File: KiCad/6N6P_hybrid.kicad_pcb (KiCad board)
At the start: 2 copper layers, 170 x 140.9 mm, 71 parts, among them J1 MID Select, J10 Screw_Terminal_01x03, J11 Screw_Terminal_01x01, J12 Screw_Terminal_01x01, J13 Screw_Terminal_01x01, J14 Screw_Terminal_01x01, J15 PSU ground, J16 Screw_Terminal_01x01, J17 center tap, J18 chassis, J2 Input, J3 MID Bypass, J4 Low boost, J5 PrePower, J6 Volume, J7 Hi Cut, J8 6N6P, J9 OT feedback, Q1 BC107, U1 LTC1151CN8, U2 LTC1151CN8

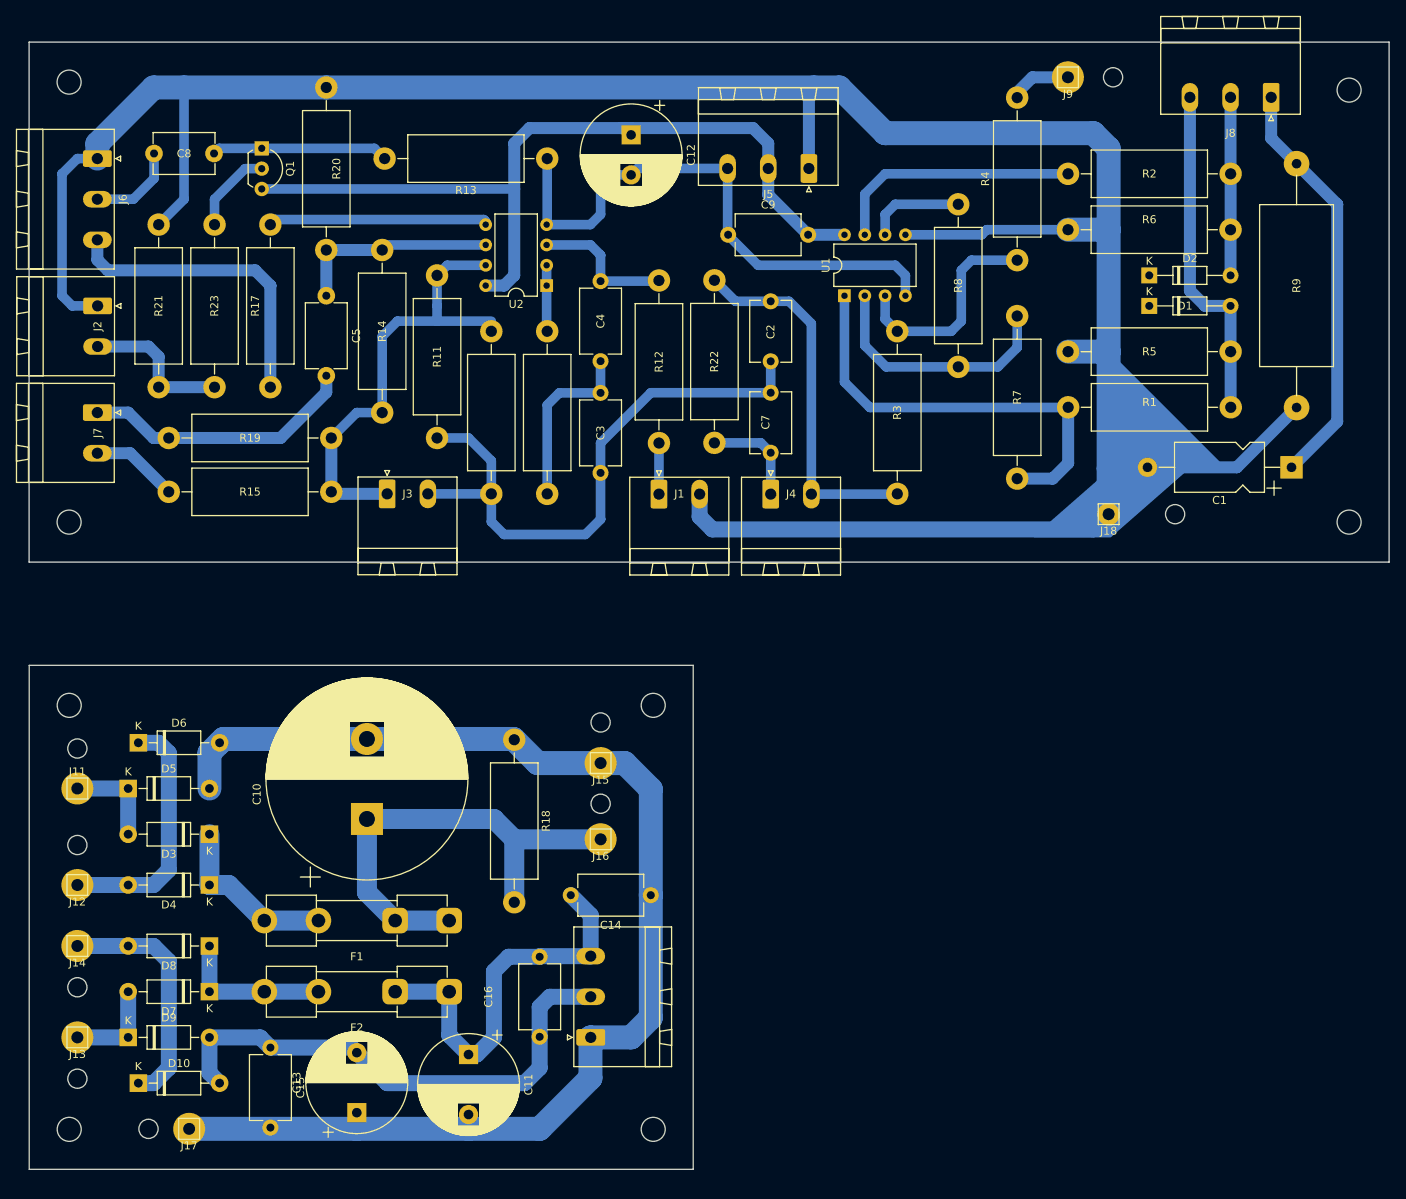
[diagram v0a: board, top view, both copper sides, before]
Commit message: Add files via upload
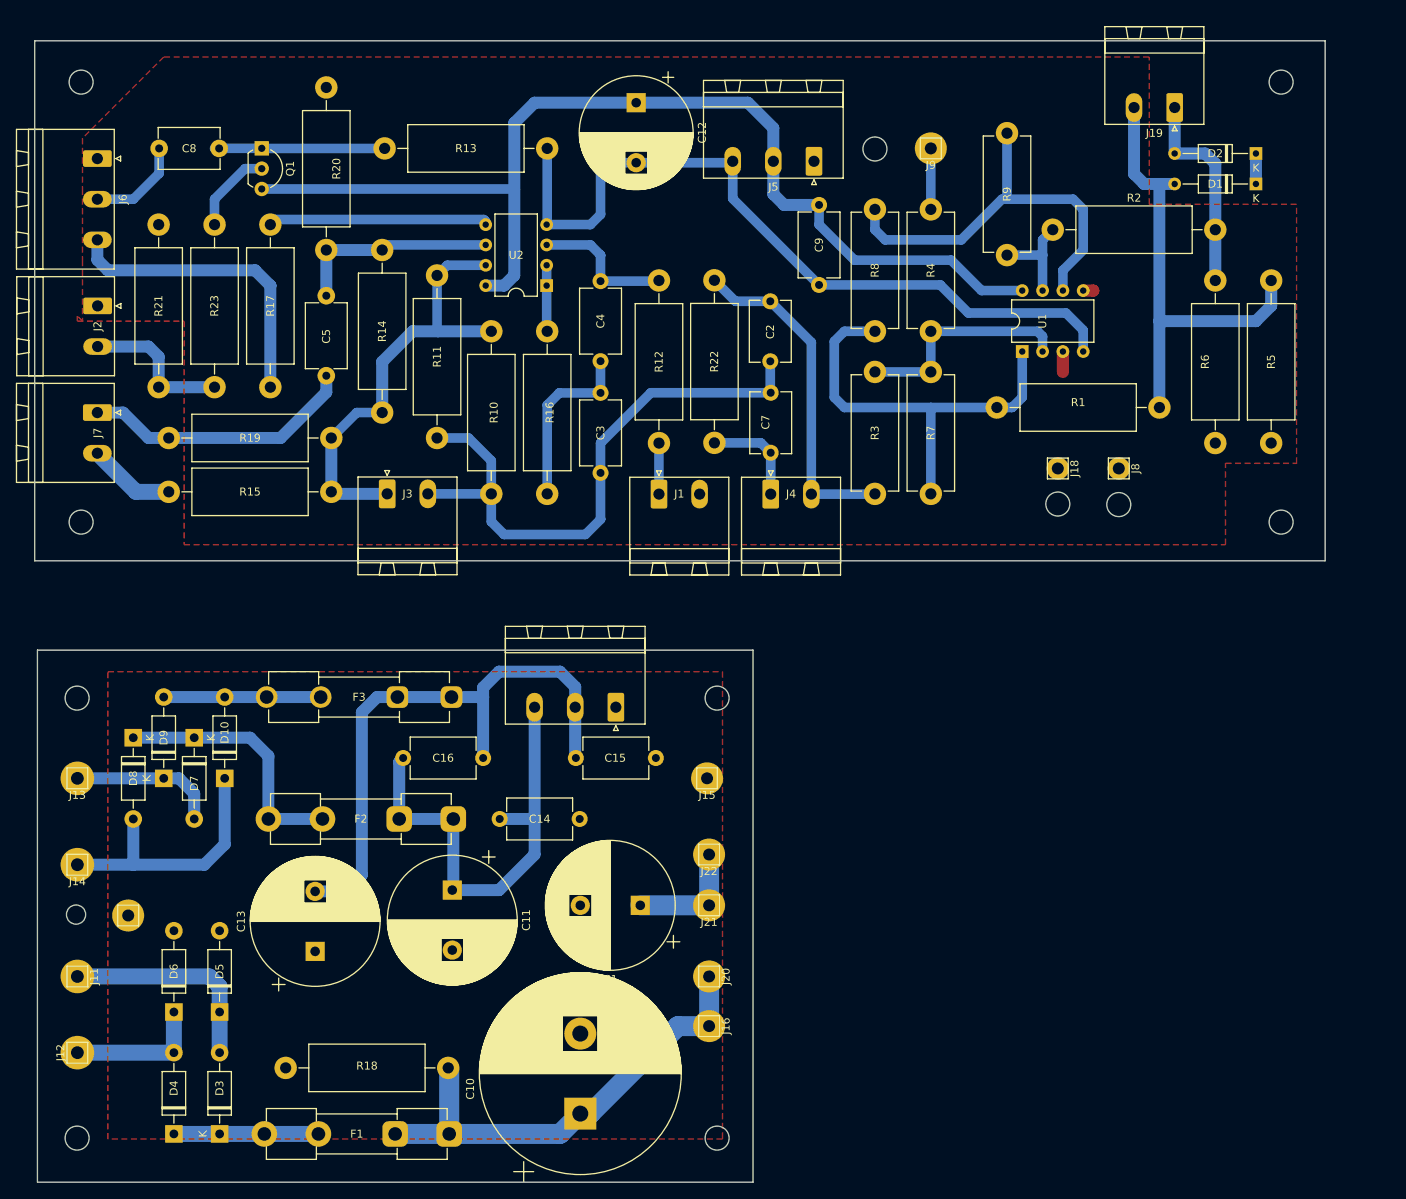
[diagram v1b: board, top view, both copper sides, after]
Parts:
- added F3: Fuse, Fuse:Fuseholder_Clip-5x20mm_Keystone_3517_Inline_P23.11x6.76mm_D1.70mm_Horizontal, F.Cu at (72.8, 102.9)
- added J19: TUBE, Connector_Phoenix_MSTB:PhoenixContact_MSTBA_2,5_2-G-5,08_1x02_P5.08mm_Horizontal, F.Cu at (163.2, 29.2)
- added J20: Screw_Terminal_01x01, Connector_Pin:Pin_D1.1mm_L8.5mm_W2.5mm_FlatFork, F.Cu at (105.0, 137.8)
- added J21: Screw_Terminal_01x01, Connector_Pin:Pin_D1.1mm_L8.5mm_W2.5mm_FlatFork, F.Cu at (105.0, 128.9)
- added J22: Screw_Terminal_01x01, Connector_Pin:Pin_D1.1mm_L8.5mm_W2.5mm_FlatFork, F.Cu at (105.0, 122.6)
- C1: value 22u -> 68u/350V; footprint Capacitor_THT:CP_Axial_L11.0mm_D6.0mm_P18.00mm_Horizontal -> Capacitor_THT:CP_Radial_D16.0mm_P7.50mm
- C11, C13: footprint Capacitor_THT:CP_Radial_D12.5mm_P7.50mm -> Capacitor_THT:CP_Radial_D16.0mm_P7.50mm
- C12: footprint Capacitor_THT:CP_Radial_D12.5mm_P5.00mm -> Capacitor_THT:CP_Radial_D14.0mm_P7.50mm
- J8: value 6N6P -> chassis; footprint Connector_Phoenix_MSTB:PhoenixContact_MSTBA_2,5_3-G-5,08_1x03_P5.08mm_Horizontal -> Connector_Pin:Pin_D1.1mm_L8.5mm_W2.5mm_FlatFork
- R3, R4, R7: footprint Resistor_THT:R_Axial_DIN0614_L14.3mm_D5.7mm_P20.32mm_Horizontal -> Resistor_THT:R_Axial_DIN0614_L14.3mm_D5.7mm_P15.24mm_Horizontal
- R8: value 12k -> 10k; footprint Resistor_THT:R_Axial_DIN0614_L14.3mm_D5.7mm_P20.32mm_Horizontal -> Resistor_THT:R_Axial_DIN0614_L14.3mm_D5.7mm_P15.24mm_Horizontal
- R9: value 390, 5W -> 10k; footprint Resistor_THT:R_Axial_DIN0922_L20.0mm_D9.0mm_P30.48mm_Horizontal -> Resistor_THT:R_Axial_DIN0614_L14.3mm_D5.7mm_P15.24mm_Horizontal
- moved C1 98.1 mm to (96.4, 128.9)
- moved C15 52.6 mm to (88.3, 110.5), turned to 0 degrees
- moved J8 50.1 mm to (156.2, 74.3), turned to 90 degrees
- moved R18 50.0 mm to (52.1, 149.2), turned to 0 degrees
- moved R9 49.9 mm to (142.2, 32.4), turned to -90 degrees
- moved C10 45.5 mm to (88.9, 154.9)
- moved J10 41.4 mm to (93.3, 104.1), turned to 180 degrees
- moved D10 39.6 mm to (44.5, 113.0), turned to 90 degrees
- moved D3 37.5 mm to (43.8, 157.5), turned to 90 degrees
- moved C16 35.6 mm to (76.8, 110.5), turned to 180 degrees
- moved D6 33.9 mm to (38.1, 142.2), turned to 90 degrees
- moved D9 32.7 mm to (36.8, 113.0), turned to 90 degrees
- moved R6 32.4 mm to (168.3, 71.1), turned to 90 degrees
- moved J13 32.4 mm to (26.0, 113.0)
- moved D7 31.8 mm to (40.6, 108.0), turned to -90 degrees
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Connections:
- C1 pad 1: Net-(J8-Pin_1) -> Net-(J21-Pin_1)
- C1 pad 2: GND -> GND2
- C13 pad 2: Net-(D10-A) -> Net-(J10-Pin_2)
- C15 pad 1: Net-(D10-A) -> Net-(J10-Pin_2)
- C16 pad 1: Net-(D10-A) -> Net-(J10-Pin_2)
- J10 pad 2: Net-(D10-A) -> Net-(J10-Pin_2)
- J8 pad 1: Net-(J8-Pin_1) -> GND
- R3 pad 1: Net-(U1A-+) -> Net-(U1A--)
- R4 pad 1: Net-(U1A-+) -> Net-(U1A--)
- R8 pad 1: Net-(U1A--) -> Net-(U1B--)
- R8 pad 2: Net-(U1B--) -> Net-(R1-Pad1)
- R9 pad 1: GND -> Net-(U1B--)
- R9 pad 2: Net-(J8-Pin_1) -> Net-(R2-Pad1)
- U1 pad 3: Net-(U1A-+) -> GND
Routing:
- net GND: track 347.1 -> 3.82 mm
- net GND2: track 161.7 -> 0.00 mm
- net Net-(J10-Pin_2): track 0.00 -> 73.9 mm
- net Net-(J8-Pin_1): track 52.0 -> 0.00 mm
- net Net-(D10-A): track 65.2 -> 19.6 mm
- net Net-(U1B--): track 12.2 -> 51.2 mm
- net V++: track 105.7 -> 135.3 mm
- net Net-(U1A-+): track 27.7 -> 0.00 mm
- net V--: track 71.2 -> 95.8 mm
- net Net-(R2-Pad1): track 31.5 -> 12.6 mm
- net Net-(D1-A): track 42.7 -> 59.8 mm
- net Net-(J21-Pin_1): track 0.00 -> 14.9 mm
- net Net-(D3-A): track 12.1 -> 26.6 mm
- net Net-(D4-A): track 31.2 -> 17.1 mm
- net Net-(D7-K): track 19.3 -> 32.5 mm
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- added copper zone on F.Cu, net GND
- added copper zone on F.Cu, net GND2
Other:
- board size 170 x 140.9 mm -> 161.3 x 142.7 mm

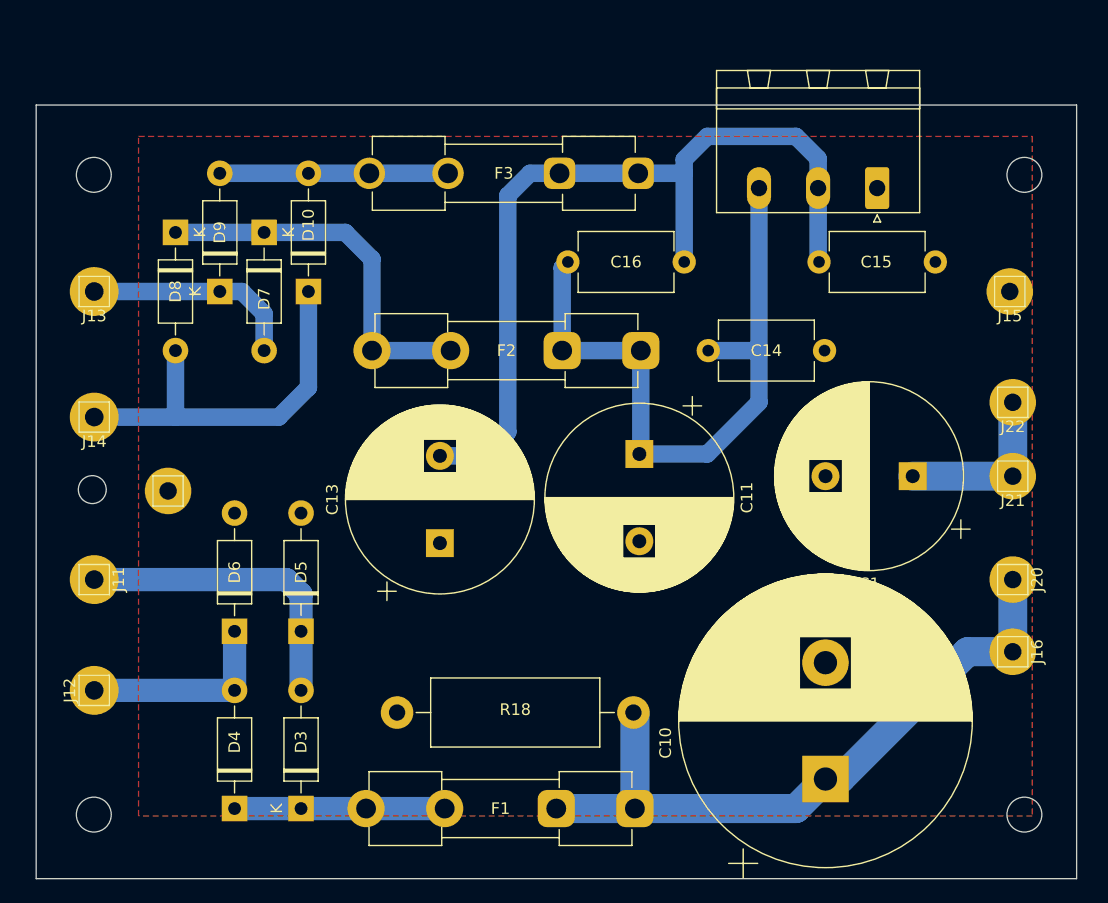
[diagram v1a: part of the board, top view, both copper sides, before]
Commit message: Add files via upload
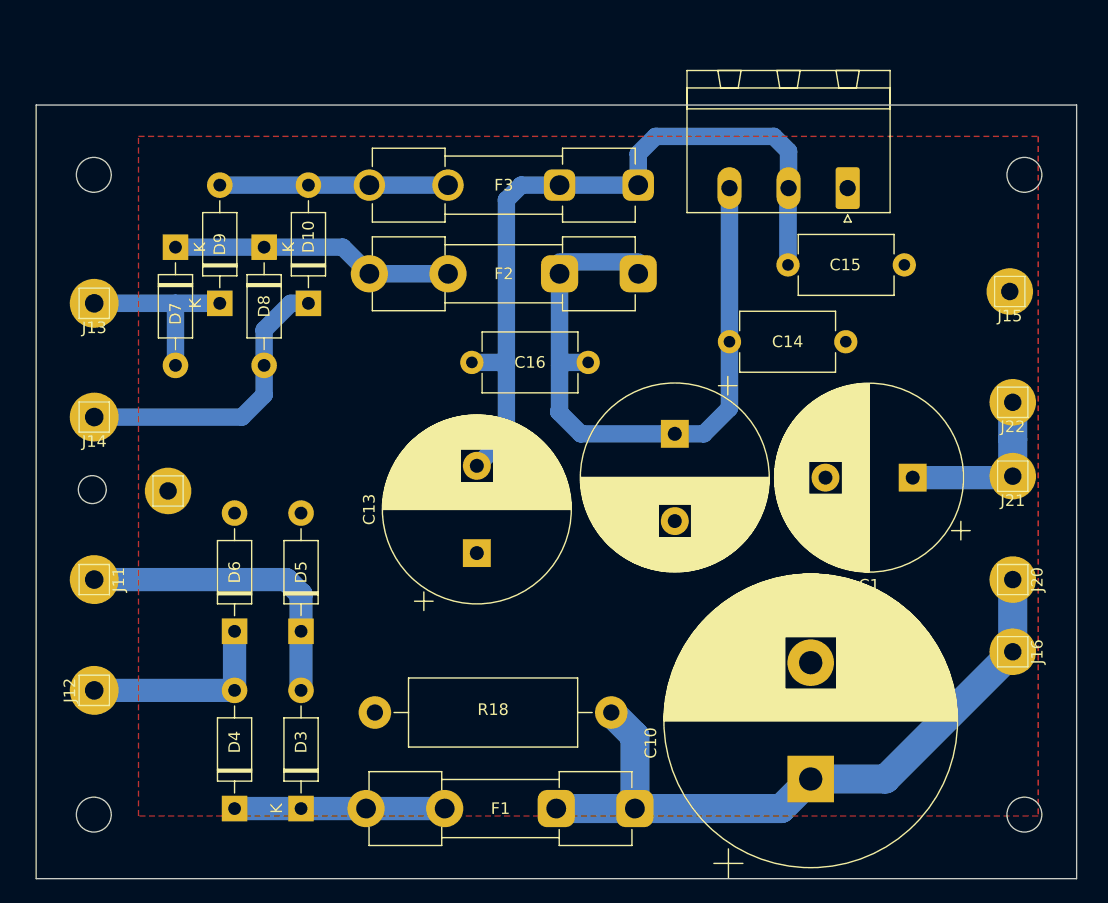
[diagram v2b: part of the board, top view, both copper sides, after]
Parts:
- moved C16 20.2 mm to (58.5, 119.1), turned to 0 degrees
- moved D7 7.73 mm to (33.0, 109.2)
- moved D8 7.73 mm to (40.6, 109.2)
- moved F2 6.61 mm to (72.8, 111.5)
- moved C11 3.51 mm to (75.9, 125.3)
- moved C13 3.29 mm to (58.9, 135.5)
- moved C15 2.68 mm to (85.7, 110.7)
- moved J10 2.54 mm to (90.8, 104.1)
- moved C14 1.98 mm to (90.6, 117.3)
- moved R18 1.91 mm to (50.2, 149.2)
- moved C10 1.27 mm to (87.6, 154.9)
- moved D10 1.02 mm to (44.5, 114.0)
- moved D9 1.02 mm to (36.8, 114.0)
- moved J13 1.02 mm to (26.0, 114.0)
- moved F3 1.02 mm to (72.8, 103.9)
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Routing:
- net Net-(J10-Pin_2): track 73.9 -> 65.4 mm
- net Net-(D7-K): track 32.5 -> 24.4 mm
- net Net-(D10-K): track 33.4 -> 25.7 mm
- net Net-(D7-A): track 18.6 -> 16.1 mm
- net Net-(J10-Pin_3): track 58.4 -> 56.5 mm
- net Net-(J16-Pin_1): track 59.5 -> 60.3 mm
